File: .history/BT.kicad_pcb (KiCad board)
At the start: 4 copper layers, 55 x 40 mm, 84 parts, among them J1 Conn_01x05_Pin, J2 Conn_01x03_Pin, J3 Conn_01x06_Pin, J5 Conn_02x03_Odd_Even, K1 AGQ200S12Z, Q1 BSS123, U1 PCM5100A, U2 ESP32-WROOM-32U, U3 TLV4888DR, U4 AP64060WU-7, U6 TPS7A4701, U7 AP64060WU-7, Y1 XO32

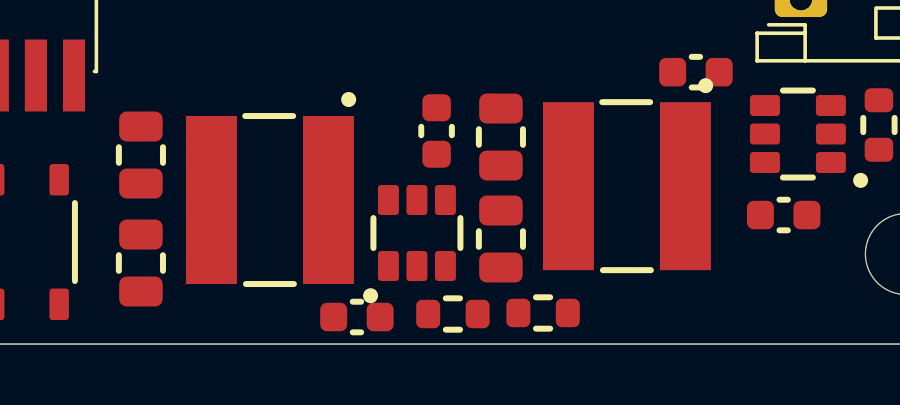
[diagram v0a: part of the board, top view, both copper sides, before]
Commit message: clean up
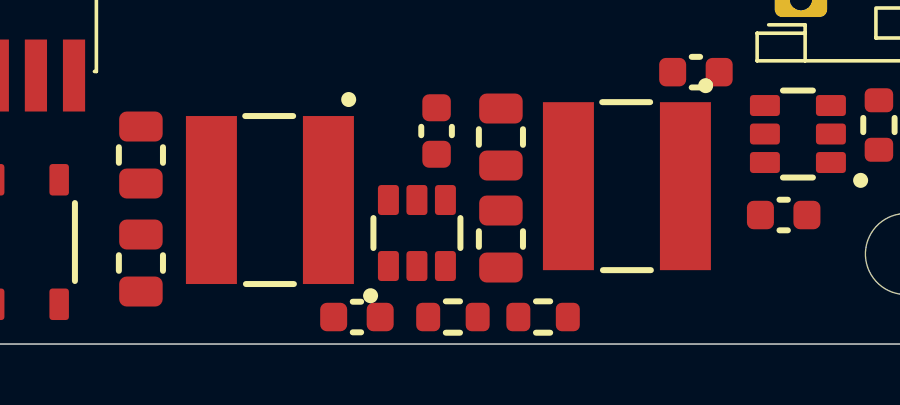
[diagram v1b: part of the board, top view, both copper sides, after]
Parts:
- moved R31 0.14 mm to (160.6, 114.8)
- moved R20 0.10 mm to (157.6, 114.8)
- turned C30 to 180 degrees
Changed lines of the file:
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@@
 	(footprint "NRD_RES:R_0603"
 		(layer "F.Cu")
-		(at 160.595 114.675)
+		(at 160.595 114.81)
 		(tags "resistor")
 		(property "Reference" "R31"
@@
 	(footprint "NRD_CAP:C_0603"
 		(layer "F.Cu")
-		(at 154.39 114.81)
+		(at 154.39 114.81 180)
 		(property "Reference" "C30"
 			(at 0 -1.43 0)
@@
 		)
 		(property "Manufacturer" "Samsung"
-			(at 0 0 0)
+			(at 0 0 180)
 			(unlocked yes)
 			(layer "F.Fab")
@@
 		)
 		(property "Manufacturer Part Number" "CL10B104KB8NNNC"
-			(at 0 0 0)
+			(at 0 0 180)
 			(unlocked yes)
 			(layer "F.Fab")
@@
 		)
 		(property "Maximum Operating Temperature [°C]" "125"
-			(at 0 0 0)
+			(at 0 0 180)
 			(unlocked yes)
 			(layer "F.Fab")
@@
 		)
 		(property "Voltage" "50V"
-			(at 0 0 0)
+			(at 0 0 180)
 			(unlocked yes)
 			(layer "F.Fab")
@@
 		)
 		(property "Voltage [V]" "50"
-			(at 0 0 0)
+			(at 0 0 180)
 			(unlocked yes)
 			(layer "F.Fab")
@@
 		)
 		(property "Minimum Operating Temperature [°C]" "-55"
-			(at 0 0 0)
+			(at 0 0 180)
 			(unlocked yes)
 			(layer "F.Fab")
@@
 		)
 		(property "Package" "0603"
-			(at 0 0 0)
+			(at 0 0 180)
 			(unlocked yes)
 			(layer "F.Fab")
@@
 		)
 		(property "RoHS" "Yes"
-			(at 0 0 0)
+			(at 0 0 180)
 			(unlocked yes)
 			(layer "F.Fab")
@@
 		)
 		(property "Tolerance" "±10%"
-			(at 0 0 0)
+			(at 0 0 180)
 			(unlocked yes)
 			(layer "F.Fab")
@@
 		)
 		(property "Tolerance [%]" "10"
-			(at 0 0 0)
+			(at 0 0 180)
 			(unlocked yes)
 			(layer "F.Fab")
@@
 		)
 		(property "Dielectric" "X7R"
-			(at 0 0 0)
+			(at 0 0 180)
 			(unlocked yes)
 			(layer "F.Fab")
@@
 		)
 		(property "Value [F]" "1e-07"
-			(at 0 0 0)
+			(at 0 0 180)
 			(unlocked yes)
 			(layer "F.Fab")
@@
 		(duplicate_pad_numbers_are_jumpers no)
 		(fp_line
-			(start -0.14058 -0.51)
-			(end 0.14058 -0.51)
+			(start -0.14058 0.51)
+			(end 0.14058 0.51)
 			(stroke
 				(width 0.2)
@@
 		)
 		(fp_line
-			(start -0.14058 0.51)
-			(end 0.14058 0.51)
+			(start -0.14058 -0.51)
+			(end 0.14058 -0.51)
 			(stroke
 				(width 0.2)
@@
 		)
 		(pad "1" smd roundrect
-			(at -0.775 0)
+			(at -0.775 0 180)
 			(size 0.9 0.95)
 			(layers "F.Cu" "F.Mask" "F.Paste")
@@
 		)
 		(pad "2" smd roundrect
-			(at 0.775 0)
+			(at 0.775 0 180)
 			(size 0.9 0.95)
 			(layers "F.Cu" "F.Mask" "F.Paste")
@@
 	(footprint "NRD_RES:R_0603"
 		(layer "F.Cu")
-		(at 157.59 114.71)
+		(at 157.59 114.81)
 		(tags "resistor")
 		(property "Reference" "R20"
